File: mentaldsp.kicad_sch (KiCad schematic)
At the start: 30 parts, among them J1 Conn_PWRJack_2x5.5mm_CUIDevic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, J5 NEMA Conn, J7 NEMA Conn, J8 NEMA Conn, U6 ESP32-S3-SUPERMINI, U7 TMC2209_N0, U8 TMC2209_N2, U9 TMC2209_N1

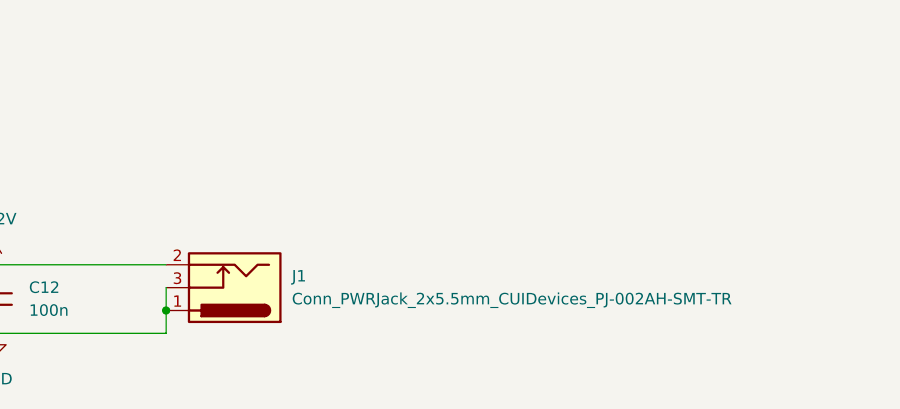
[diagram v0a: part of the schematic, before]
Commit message: fix polarity
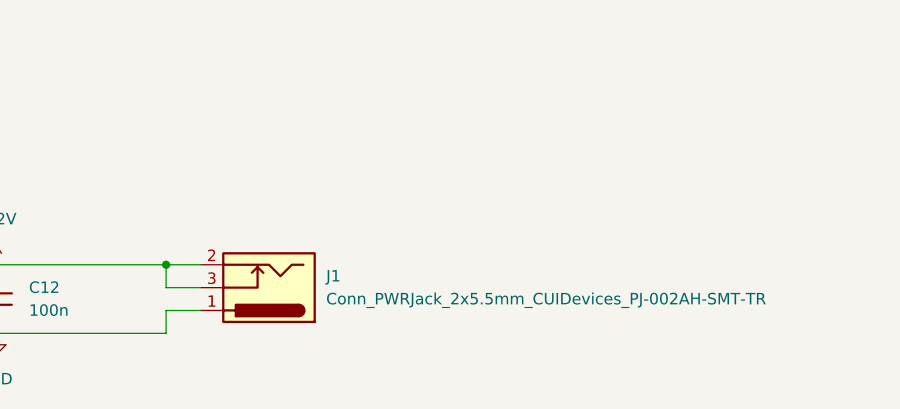
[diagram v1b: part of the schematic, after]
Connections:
- net +12V: now also J1.3
- net GND: no longer J1.3
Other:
- moved on the sheet: J1
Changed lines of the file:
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@@
 	)
 	(junction
-		(at 233.68 143.51)
+		(at 252.73 143.51)
 		(diameter 0)
 		(color 0 0 0 0)
 	)
 	(junction
-		(at 179.07 38.1)
+		(at 233.68 143.51)
 		(diameter 0)
 		(color 0 0 0 0)
 	)
 	(junction
-		(at 171.45 107.95)
+		(at 179.07 38.1)
 		(diameter 0)
 		(color 0 0 0 0)
 	)
 	(junction
-		(at 252.73 148.59)
+		(at 171.45 107.95)
 		(diameter 0)
 		(color 0 0 0 0)
@@
 	(wire
 		(pts
-			(xy 252.73 146.05) (xy 252.73 148.59)
-		)
-		(stroke
-			(width 0)
-			(type default)
-		)
-	)
-	(wire
-		(pts
 			(xy 166.37 73.66) (xy 171.45 73.66)
 		)
@@
 	(wire
 		(pts
+			(xy 256.54 146.05) (xy 252.73 146.05)
+		)
+		(stroke
+			(width 0)
+			(type default)
+		)
+	)
+	(wire
+		(pts
 			(xy 58.42 58.42) (xy 64.77 58.42)
 		)
@@
 	(wire
 		(pts
+			(xy 252.73 143.51) (xy 256.54 143.51)
+		)
+		(stroke
+			(width 0)
+			(type default)
+		)
+	)
+	(wire
+		(pts
 			(xy 113.03 130.81) (xy 132.08 130.81)
 		)
@@
 	(wire
 		(pts
+			(xy 256.54 148.59) (xy 252.73 148.59)
+		)
+		(stroke
+			(width 0)
+			(type default)
+		)
+	)
+	(wire
+		(pts
 			(xy 167.64 130.81) (xy 171.45 130.81)
 		)
@@
 	(wire
 		(pts
+			(xy 252.73 146.05) (xy 252.73 143.51)
+		)
+		(stroke
+			(width 0)
+			(type default)
+		)
+	)
+	(wire
+		(pts
 			(xy 41.91 63.5) (xy 41.91 67.31)
 		)
@@
 	(symbol
 		(lib_id "PCM_fab:Conn_PWRJack_2x5.5mm_CUIDevices_PJ-002AH-SMT-TR")
-		(at 260.35 146.05 180)
+		(at 264.16 146.05 180)
 		(unit 1)
 		(body_style 1)
@@
 		(fields_autoplaced yes)
 		(property "Reference" "J1"
-			(at 266.7 144.7799 0)
+			(at 270.51 144.7799 0)
 			(show_name no)
 			(do_not_autoplace no)
@@
 		)
 		(property "Value" "Conn_PWRJack_2x5.5mm_CUIDevices_PJ-002AH-SMT-TR"
-			(at 266.7 147.3199 0)
+			(at 270.51 147.3199 0)
 			(show_name no)
 			(do_not_autoplace no)
@@
 		)
 		(property "Footprint" "PCM_fab:CUIDevices_PJ-002AH-SMT-TR_PWRJack_2x5.5mm"
-			(at 259.08 145.034 0)
+			(at 262.89 145.034 0)
 			(hide yes)
 			(show_name no)
@@
 		)
 		(property "Datasheet" "https://www.cuidevices.com/product/resource/pj-002ah-smt-tr.pdf"
-			(at 259.08 145.034 0)
+			(at 262.89 145.034 0)
 			(hide yes)
 			(show_name no)
@@
 		)
 		(property "Description" "Power Barrel Connector Jack 2.00mm ID (0.079\"), 5.50mm OD (0.217\") Surface Mount"
-			(at 260.35 146.05 0)
+			(at 264.16 146.05 0)
 			(hide yes)
 			(show_name no)
